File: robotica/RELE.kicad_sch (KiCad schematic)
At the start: 18 parts, among them J7 salidas, K3 FINDER-36.11, Q9 2N3904, U11 4N35

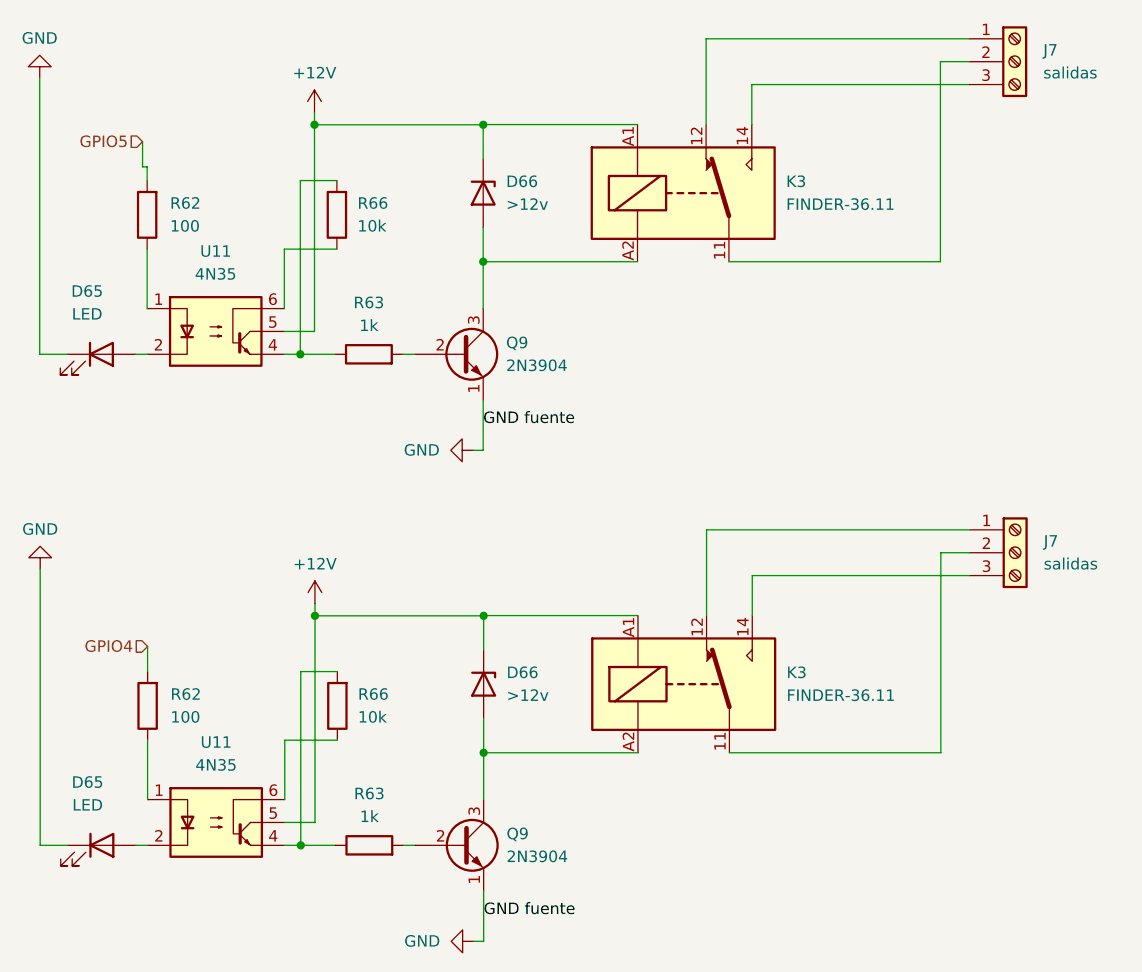
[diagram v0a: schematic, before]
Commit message: PCB YA REALIZADO
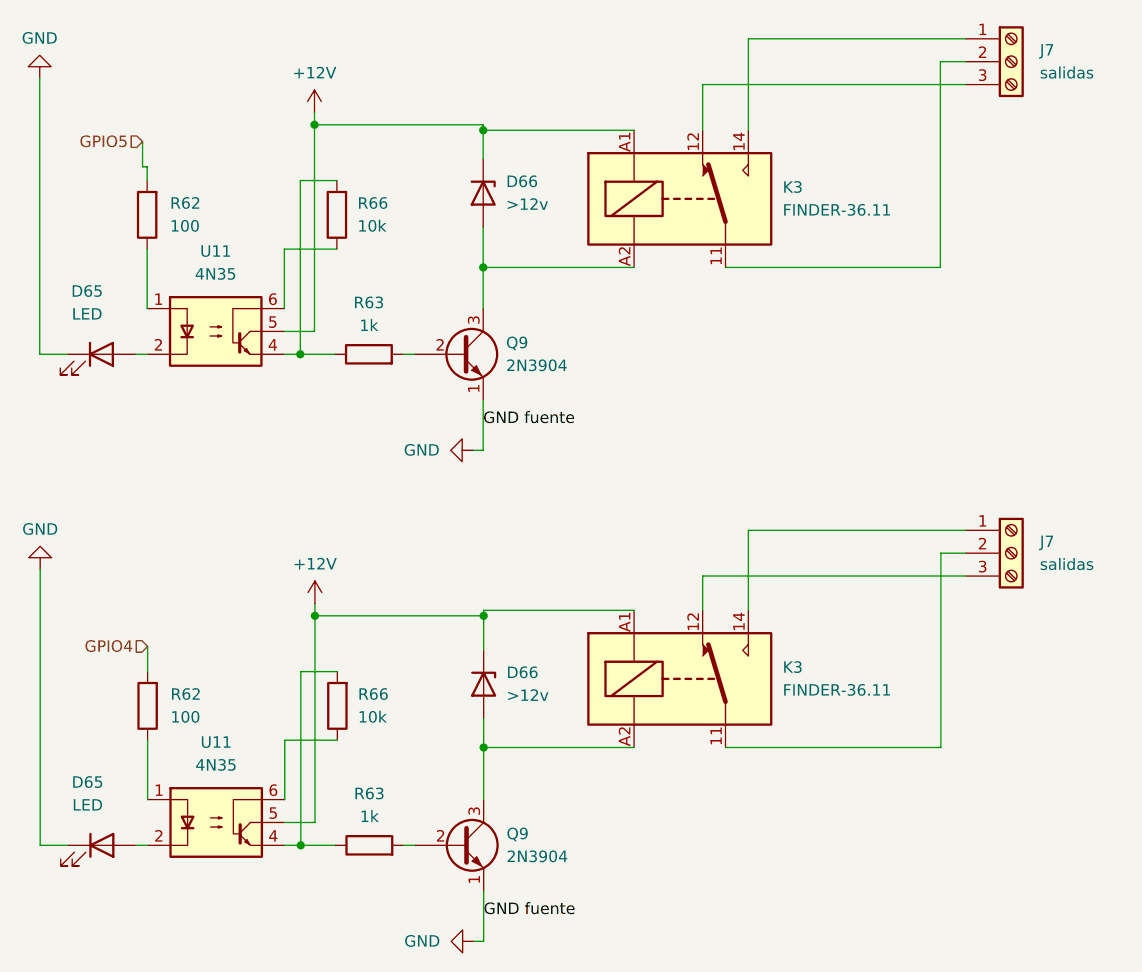
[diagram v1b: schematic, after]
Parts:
- R62, R63, R66: footprint Resistor_THT:R_Axial_DIN0207_L6.3mm_D2.5mm_P10.16mm_Horizontal -> Resistor_THT:R_Axial_DIN0207_L6.3mm_D2.5mm_P7.62mm_Horizontal
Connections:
- net at K3.12: now also J7.3 (Pin_3); no longer J7.1 (Pin_1)
- net at K3.14: now also J7.1 (Pin_1); no longer J7.3 (Pin_3)
- net at J7.1 (Pin_1): now also K3.14; no longer K3.12
- net at J7.3 (Pin_3): now also K3.12; no longer K3.14
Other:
- moved on the sheet: K3
